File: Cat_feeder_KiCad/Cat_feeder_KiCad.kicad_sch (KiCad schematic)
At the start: 18 parts, among them J1 Conn_01x03_Pin, SW1 SW_Push, SW2 Reset button, U1 ESP32-S3-WROOM-1, U2 DS3231M, U3 ER_OLEDM0.91_1x-I2C, U4 LD1117V33

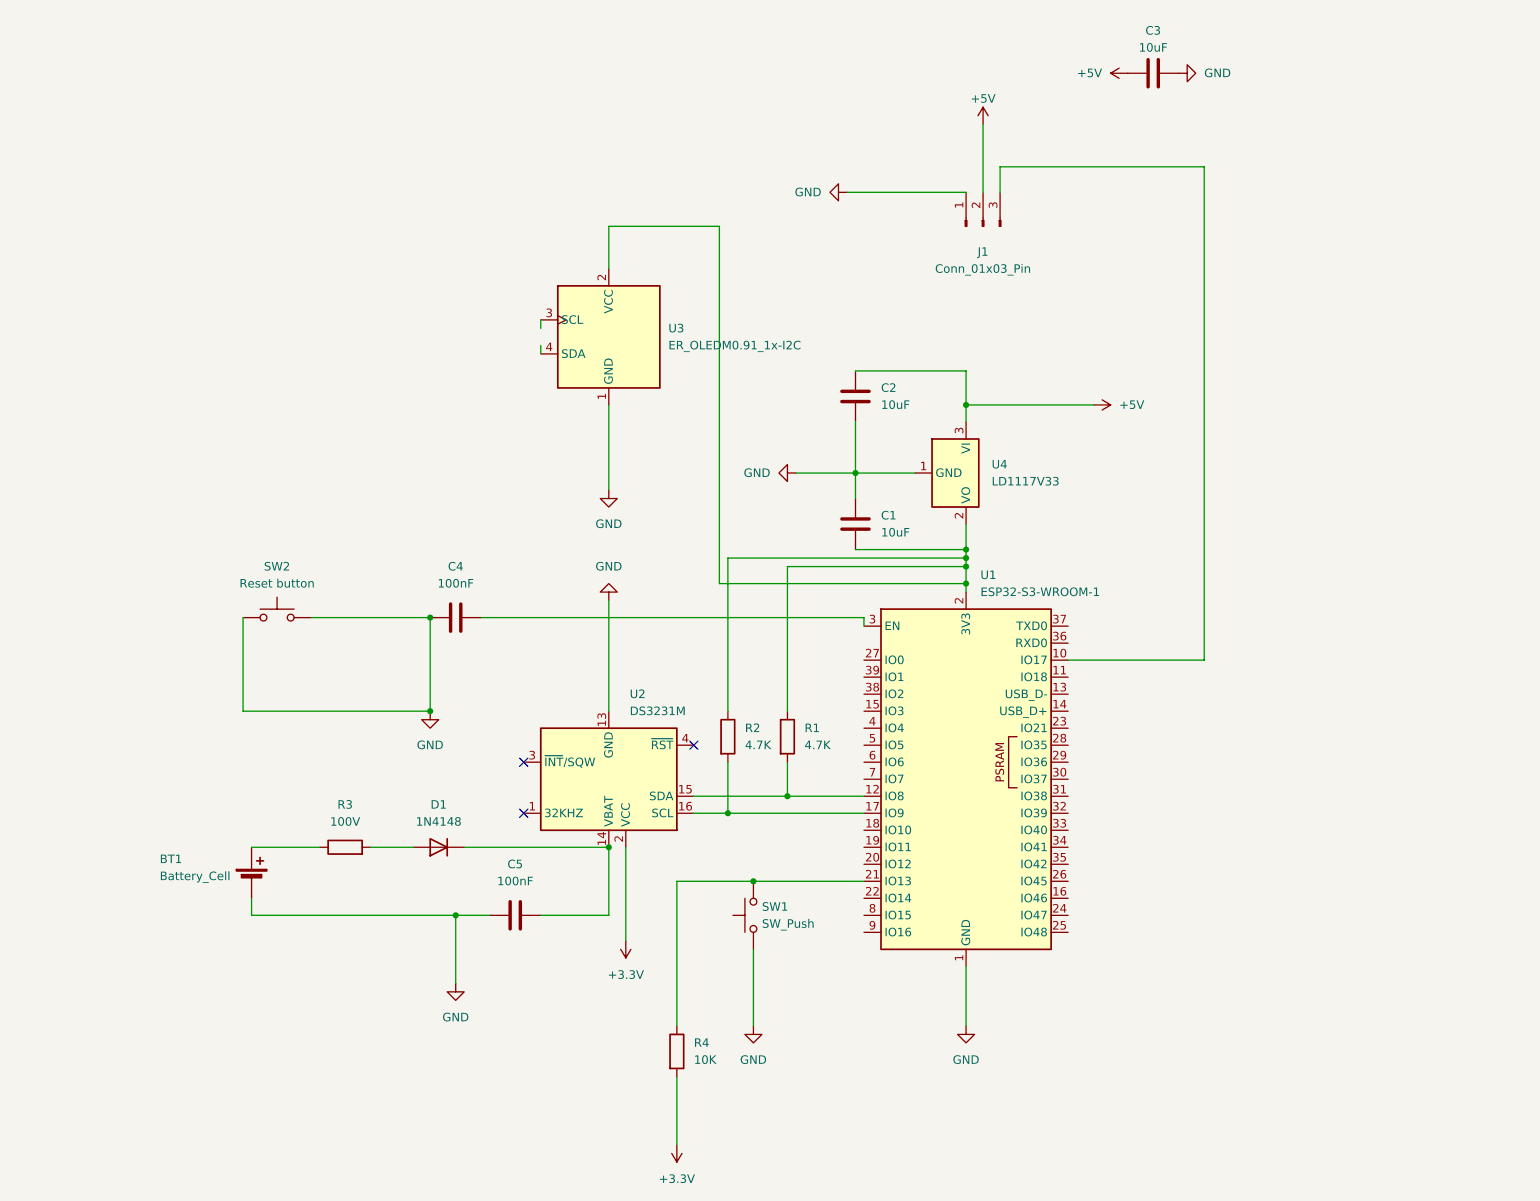
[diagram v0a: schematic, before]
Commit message: polishing and editing schematic
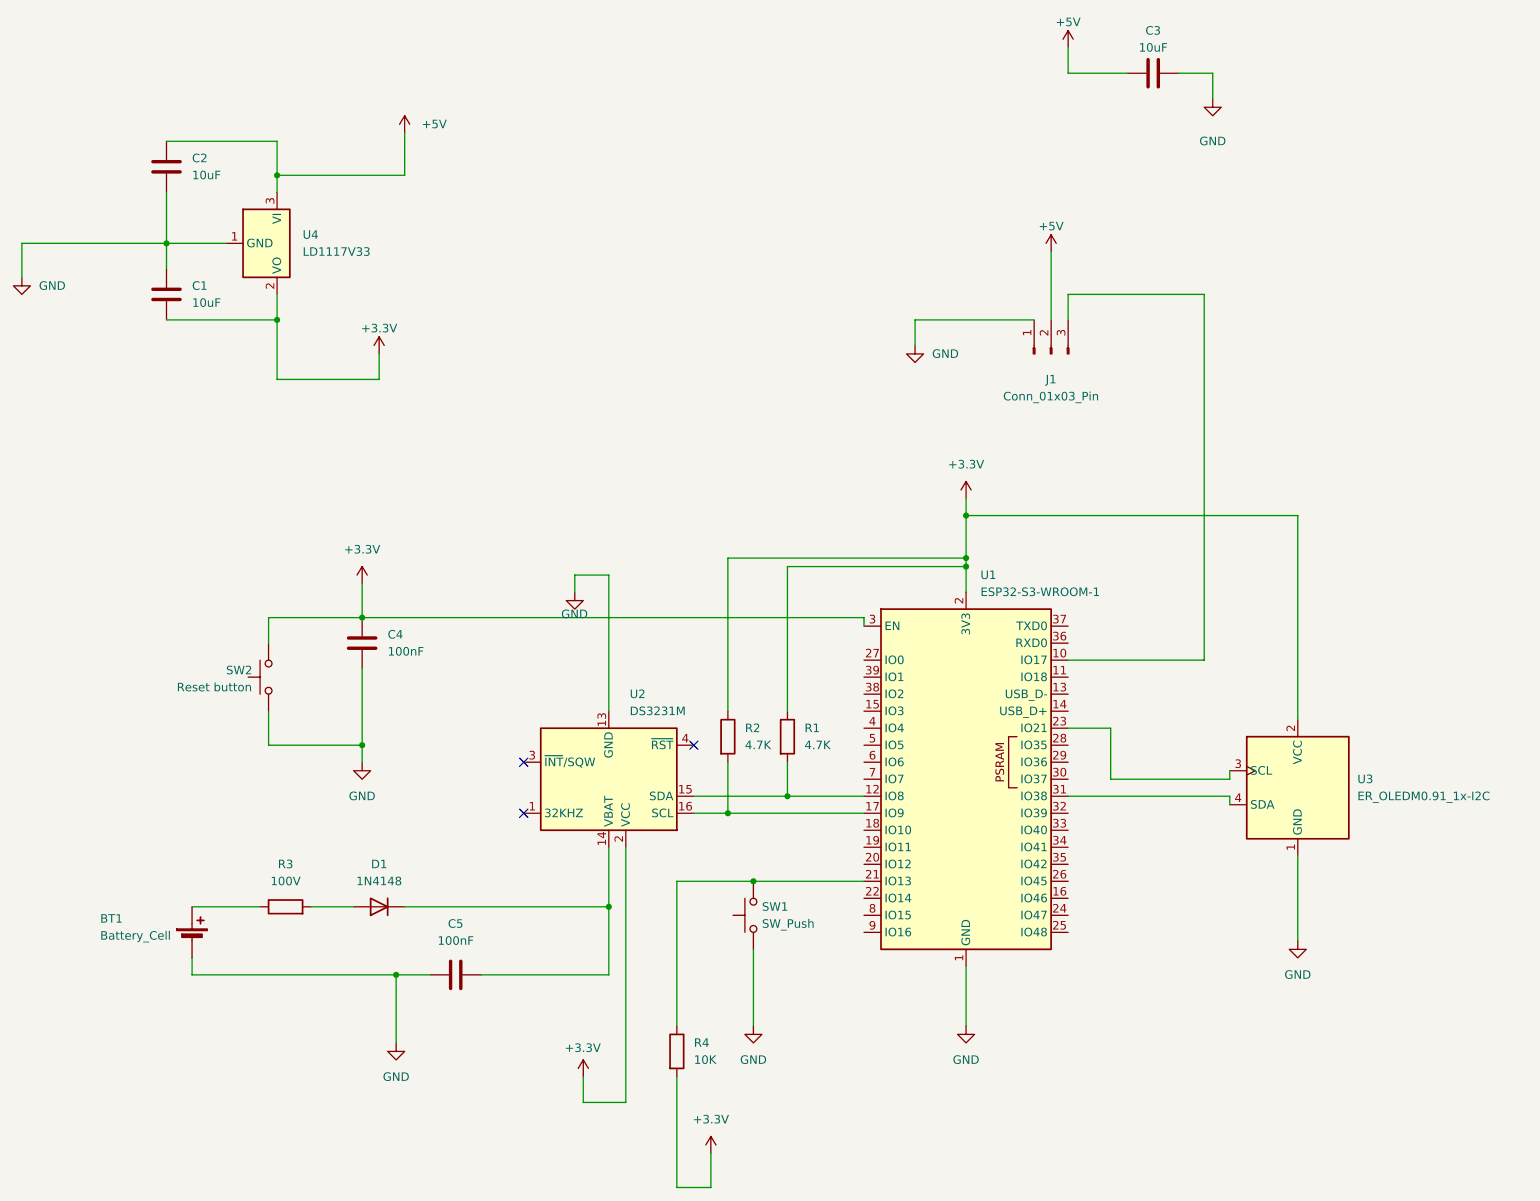
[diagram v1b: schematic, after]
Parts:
- BT1: footprint (none) -> Battery:BatteryHolder_Keystone_3034_1x20mm
- SW2: footprint (none) -> Button_Switch_THT:SW_PUSH_6mm
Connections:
- net +3.3V: now also C1.2, C4.1, R1.1, R2.1, SW2.2, U1.2 (3V3), U1.3 (EN), U3.2 (VCC), U4.2 (VO)
- net GND: no longer SW2.2
- net at U3.3 (SCL): now also U1.23 (IO21)
- net at U3.4 (SDA): now also U1.31 (IO38)
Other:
- moved on the sheet: BT1, C1, C2, C4, C5, D1, J1, R3, SW2, U3, U4
